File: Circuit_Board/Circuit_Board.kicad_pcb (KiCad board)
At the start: 2 copper layers, 67.3 x 56 mm, 17 parts, among them J1 Conn_01x02, J2 Control stuff, J3 Power stuff, J4 Conn_02x06_Odd_Even, U1 Pico

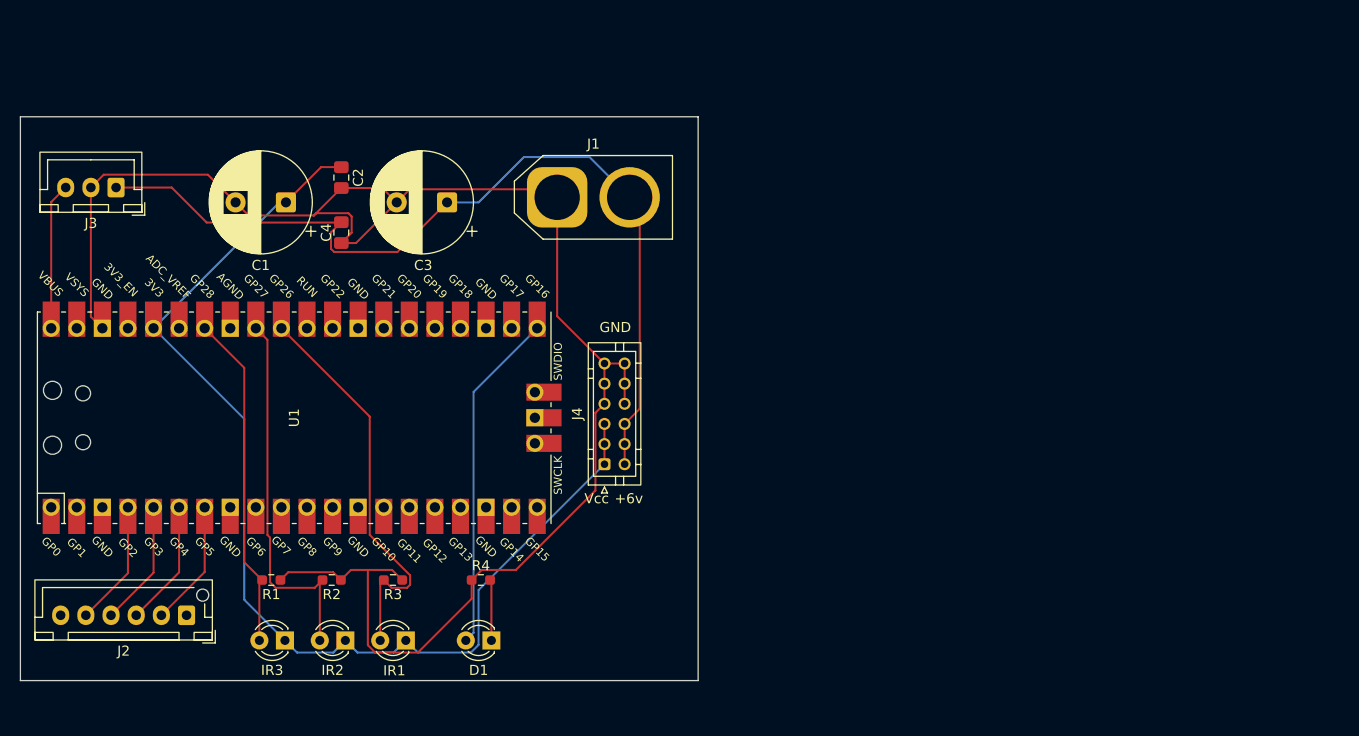
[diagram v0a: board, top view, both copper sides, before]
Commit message: Changed board design
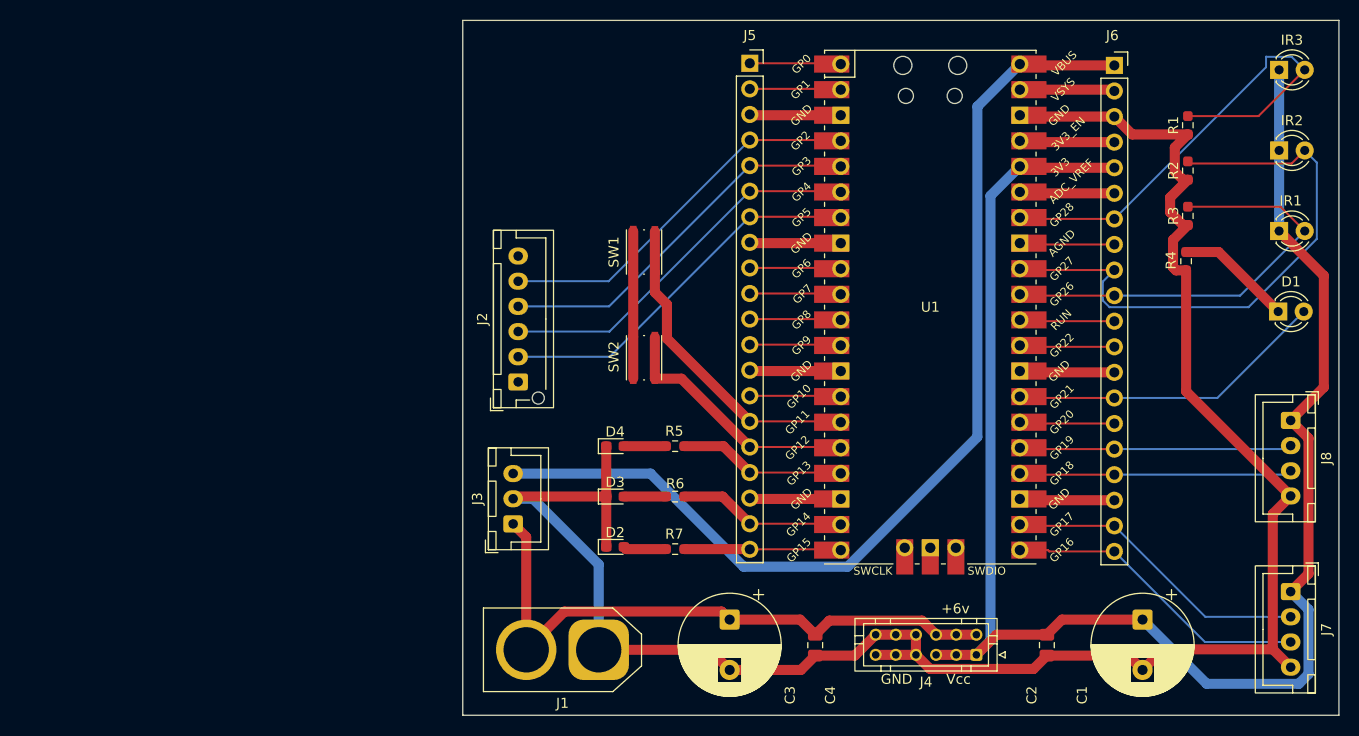
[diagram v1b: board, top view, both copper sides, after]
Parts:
- added D2: LED, LED_SMD:LED_0603_1608Metric_Pad1.05x0.95mm_HandSolder, F.Cu at (117.6, 119.2)
- added D3: LED, LED_SMD:LED_0603_1608Metric_Pad1.05x0.95mm_HandSolder, F.Cu at (117.6, 114.2)
- added D4: LED, LED_SMD:LED_0603_1608Metric_Pad1.05x0.95mm_HandSolder, F.Cu at (117.6, 109.2)
- added J5: Conn_01x20_Socket, Connector_PinSocket_2.54mm:PinSocket_1x20_P2.54mm_Vertical, F.Cu at (130.9, 71.2)
- added J6: Conn_01x20_Socket, Connector_PinSocket_2.54mm:PinSocket_1x20_P2.54mm_Vertical, F.Cu at (167.1, 71.4)
- added J7: Conn_01x04_Socket, Connector_JST:JST_XH_B4B-XH-A_1x04_P2.50mm_Vertical, F.Cu at (184.6, 123.7)
- added J8: Conn_01x04_Socket, Connector_JST:JST_XH_B4B-XH-A_1x04_P2.50mm_Vertical, F.Cu at (184.6, 106.7)
- added R5: R, Resistor_SMD:R_0603_1608Metric_Pad0.98x0.95mm_HandSolder, F.Cu at (123.5, 109.2)
- added R6: R, Resistor_SMD:R_0603_1608Metric_Pad0.98x0.95mm_HandSolder, F.Cu at (123.5, 114.2)
- added R7: R, Resistor_SMD:R_0603_1608Metric_Pad0.98x0.95mm_HandSolder, F.Cu at (123.5, 119.4)
- added SW1: SW_Push, Button_Switch_SMD:SW_Push_1P1T_NO_Vertical_Wuerth_434133025816, F.Cu at (120.4, 89.9)
- added SW2: SW_Push, Button_Switch_SMD:SW_Push_1P1T_NO_Vertical_Wuerth_434133025816, F.Cu at (120.4, 100.4)
- moved IR3 113.8 mm to (183.5, 71.8), turned to 0 degrees
- moved IR2 104.7 mm to (183.5, 79.8), turned to 0 degrees
- moved R1 101.6 mm to (174.4, 77.3), turned to 90 degrees
- moved IR1 95.8 mm to (183.5, 87.8), turned to 0 degrees
- moved C1 94.6 mm to (169.9, 126.4), turned to -90 degrees
- moved R2 94.2 mm to (174.4, 81.8), turned to 90 degrees
- moved R3 86.8 mm to (174.4, 86.3), turned to 90 degrees
- moved D1 84.7 mm to (183.4, 95.8), turned to 0 degrees
- moved C2 84.0 mm to (160.4, 129.0)
- moved R4 76.9 mm to (174.3, 90.8), turned to 90 degrees
- moved U1 64.1 mm to (148.9, 95.4), turned to 0 degrees
- moved C4 62.4 mm to (137.4, 129.0)
- moved J3 51.7 mm to (107.4, 116.9), turned to 90 degrees
- moved C3 50.0 mm to (128.9, 126.4), turned to -90 degrees
- moved J1 45.1 mm to (115.9, 129.4), turned to 180 degrees
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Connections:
- U1 pad 1: unconnected-(U1-GPIO0-Pad1) -> Net-(J5-Pin_1)
- U1 pad 10: unconnected-(U1-GPIO7-Pad10) -> Net-(J5-Pin_10)
- U1 pad 11: unconnected-(U1-GPIO8-Pad11) -> Net-(J5-Pin_11)
- U1 pad 12: unconnected-(U1-GPIO9-Pad12) -> Net-(J5-Pin_12)
- U1 pad 13: unconnected-(U1-GND-Pad13) -> Net-(J5-Pin_13)
- U1 pad 14: unconnected-(U1-GPIO10-Pad14) -> Net-(J5-Pin_14)
- U1 pad 15: unconnected-(U1-GPIO11-Pad15) -> Net-(J5-Pin_15)
- U1 pad 16: unconnected-(U1-GPIO12-Pad16) -> Net-(J5-Pin_16)
- U1 pad 17: unconnected-(U1-GPIO13-Pad17) -> Net-(J5-Pin_17)
- U1 pad 18: unconnected-(U1-GND-Pad18) -> Net-(J5-Pin_18)
- U1 pad 19: unconnected-(U1-GPIO14-Pad19) -> Net-(J5-Pin_19)
- U1 pad 2: unconnected-(U1-GPIO1-Pad2) -> Net-(J5-Pin_2)
- U1 pad 20: unconnected-(U1-GPIO15-Pad20) -> Net-(J5-Pin_20)
- U1 pad 21: Net-(D1-A) -> Net-(J6-Pin_20)
- U1 pad 22: unconnected-(U1-GPIO17-Pad22) -> Net-(J6-Pin_19)
- U1 pad 23: unconnected-(U1-GND-Pad23) -> Net-(J6-Pin_18)
- U1 pad 24: unconnected-(U1-GPIO18-Pad24) -> Net-(J6-Pin_17)
- U1 pad 25: unconnected-(U1-GPIO19-Pad25) -> Net-(J6-Pin_16)
- U1 pad 26: unconnected-(U1-GPIO20-Pad26) -> Net-(J6-Pin_15)
- U1 pad 27: unconnected-(U1-GPIO21-Pad27) -> Net-(D1-A)
- U1 pad 28: unconnected-(U1-GND-Pad28) -> Net-(J6-Pin_13)
- U1 pad 29: unconnected-(U1-GPIO22-Pad29) -> Net-(J6-Pin_12)
- U1 pad 3: unconnected-(U1-GND-Pad3) -> Net-(J5-Pin_3)
- U1 pad 30: unconnected-(U1-RUN-Pad30) -> Net-(J6-Pin_11)
- U1 pad 33: unconnected-(U1-AGND-Pad33) -> Net-(J6-Pin_8)
- U1 pad 35: unconnected-(U1-ADC_VREF-Pad35) -> Net-(J6-Pin_6)
- U1 pad 37: unconnected-(U1-3V3_EN-Pad37) -> Net-(J6-Pin_4)
- U1 pad 39: unconnected-(U1-VSYS-Pad39) -> Net-(J6-Pin_2)
- U1 pad 8: unconnected-(U1-GND-Pad8) -> Net-(J5-Pin_8)
- U1 pad 9: unconnected-(U1-GPIO6-Pad9) -> Net-(J5-Pin_9)
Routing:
- net VBUS: track 14.6 -> 103.7 mm
- net VCC: track 110.8 -> 166.7 mm
- net Net-(J5-Pin_15): track 0.00 -> 31.8 mm
- net Net-(J6-Pin_19): track 0.00 -> 30.7 mm
- net Net-(J6-Pin_20): track 0.00 -> 30.7 mm
- net GND: track 168.9 -> 198.0 mm
- net +6V: track 89.8 -> 61.4 mm
- net Net-(J6-Pin_17): track 0.00 -> 27.1 mm
- net Net-(J6-Pin_16): track 0.00 -> 27.1 mm
- net Net-(J5-Pin_16): track 0.00 -> 25.4 mm
- net Net-(J2-Pin_5): track 12.5 -> 37.9 mm
- net Net-(J2-Pin_4): track 12.5 -> 37.9 mm
- net Net-(J2-Pin_3): track 12.5 -> 37.8 mm
- net Net-(J2-Pin_2): track 12.5 -> 37.8 mm
- net Net-(J6-Pin_9): track 37.7 -> 59.0 mm
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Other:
- board size 67.3 x 56 mm -> 87 x 69 mm
